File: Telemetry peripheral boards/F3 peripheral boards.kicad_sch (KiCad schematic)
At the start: 34 parts, among them J1 Hall Effect Sensor, J2 105313-1108, J3 Potentiometer, J4 Strain Gauge, U1 INA125U

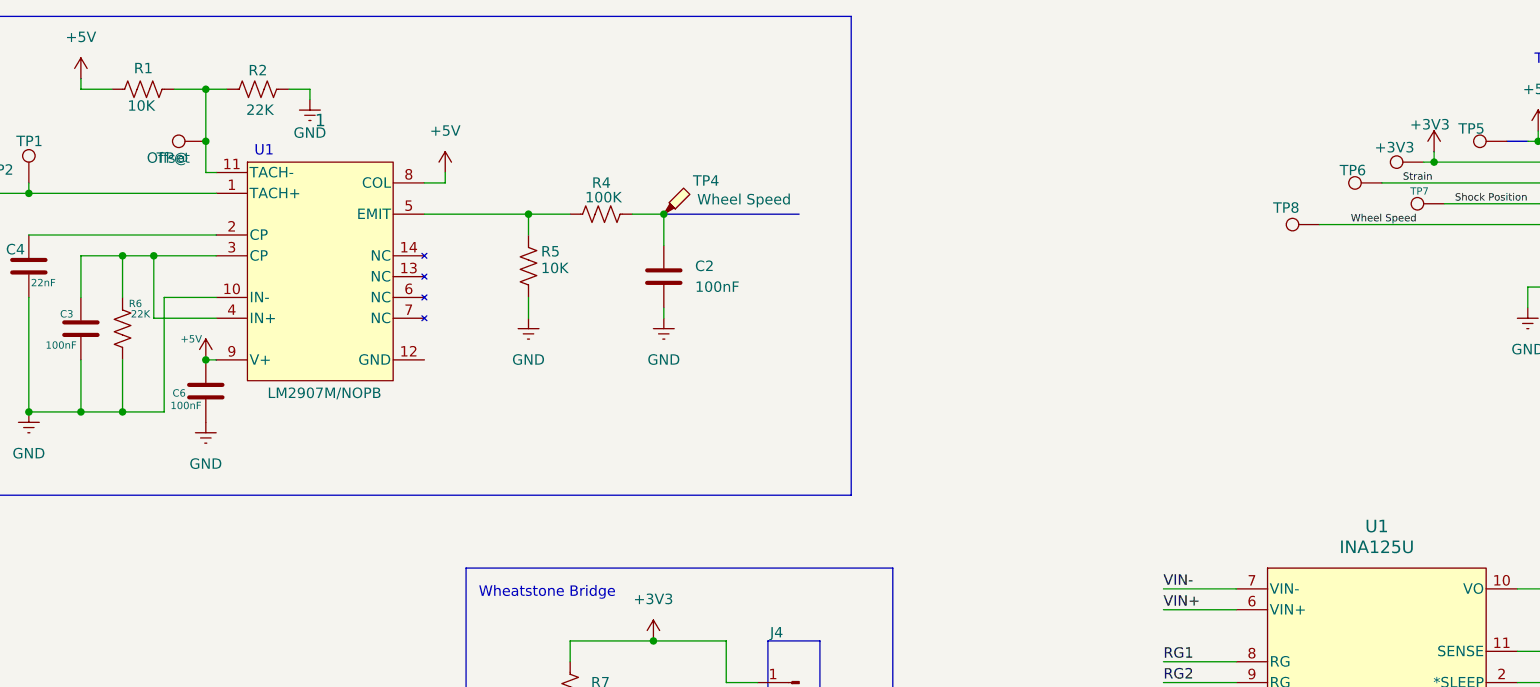
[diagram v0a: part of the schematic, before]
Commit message: Peripheral Board updates
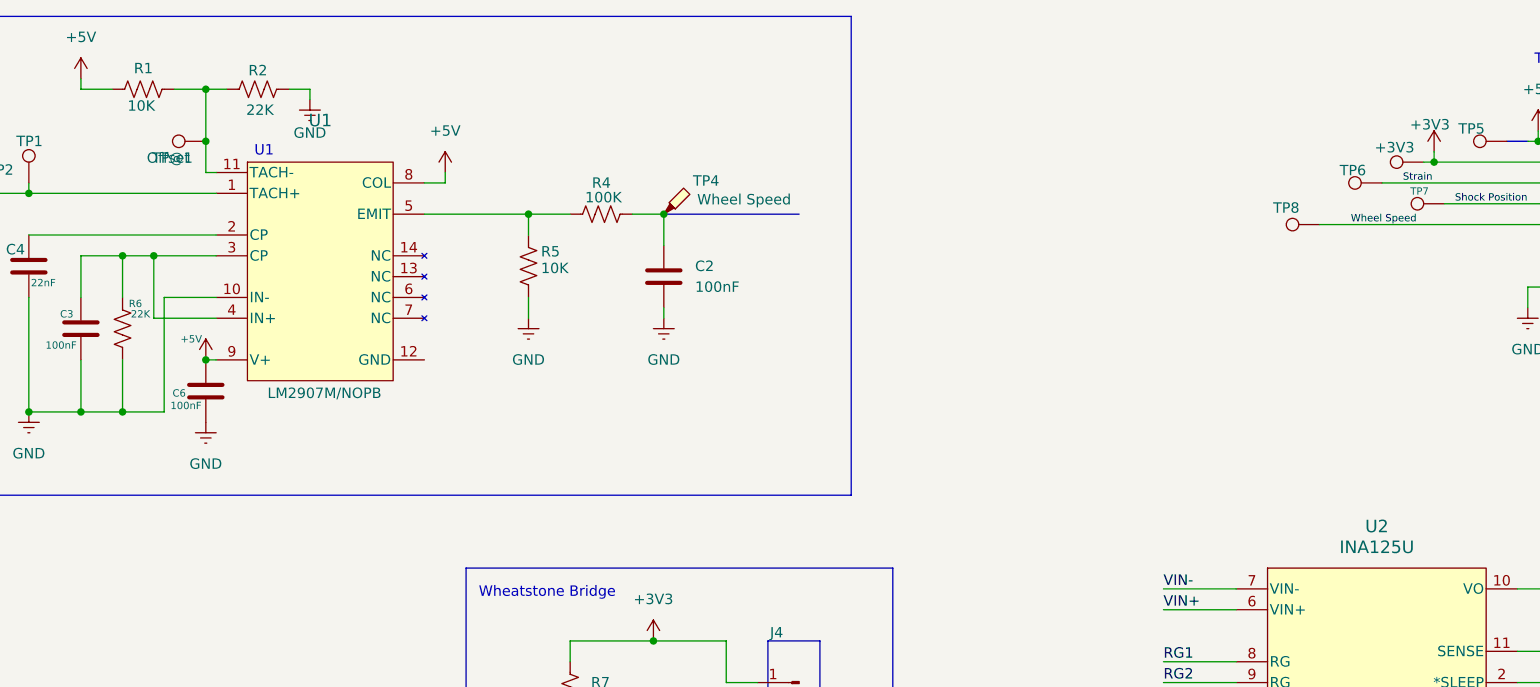
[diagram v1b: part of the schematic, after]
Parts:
- C1, C2, C3, C4, C5, C6: footprint (none) -> Capacitor_SMD:C_0805_2012Metric_Pad1.18x1.45mm_HandSolder
- R1, R10, R11, R2, R3, R4, R5, R6, R7, R8, R9: footprint (none) -> Resistor_SMD:R_0805_2012Metric_Pad1.20x1.40mm_HandSolder
- U1: renamed from 1; footprint (none) -> New Library:LM2907MNOPB
- U2: renamed from U1; footprint (none) -> New Library:105313-1108
- renumbered TP@ to TP@1
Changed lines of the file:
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@@
 			)
 		)
-		(property "Footprint" ""
+		(property "Footprint" "Resistor_SMD:R_0805_2012Metric_Pad1.20x1.40mm_HandSolder"
 			(at 94.234 30.734 90)
 			(effects
@@
 			)
 		)
-		(property "Footprint" ""
+		(property "Footprint" "Capacitor_SMD:C_0805_2012Metric_Pad1.18x1.45mm_HandSolder"
 			(at 73.3552 64.77 0)
 			(effects
@@
 			)
 		)
-		(property "Footprint" ""
+		(property "Footprint" "Resistor_SMD:R_0805_2012Metric_Pad1.20x1.40mm_HandSolder"
 			(at 78.486 61.214 90)
 			(effects
@@
 		(on_board yes)
 		(dnp no)
-		(property "Reference" "TP@"
+		(property "Reference" "TP@1"
 			(at 83.566 40.132 90)
 			(effects
@@
 			(project ""
 				(path "/dca14ea9-6ab5-4637-ab7d-1bf40ef85725"
-					(reference "TP@")
+					(reference "TP@1")
 					(unit 1)
 				)
@@
 			)
 		)
-		(property "Footprint" ""
+		(property "Footprint" "Capacitor_SMD:C_0805_2012Metric_Pad1.18x1.45mm_HandSolder"
 			(at 58.1152 57.15 0)
 			(effects
@@
 			)
 		)
-		(property "Footprint" ""
+		(property "Footprint" "Resistor_SMD:R_0805_2012Metric_Pad1.20x1.40mm_HandSolder"
 			(at 152.146 118.364 90)
 			(effects
@@
 			)
 		)
-		(property "Footprint" ""
+		(property "Footprint" "Resistor_SMD:R_0805_2012Metric_Pad1.20x1.40mm_HandSolder"
 			(at 44.196 52.324 90)
 			(effects
@@
 			)
 		)
-		(property "Footprint" ""
+		(property "Footprint" "Capacitor_SMD:C_0805_2012Metric_Pad1.18x1.45mm_HandSolder"
 			(at 67.0052 57.15 0)
 			(effects
@@
 		(dnp no)
 		(fields_autoplaced yes)
-		(property "Reference" "U1"
+		(property "Reference" "U2"
 			(at 230.505 85.09 0)
 			(effects
@@
 			)
 		)
-		(property "Footprint" ""
+		(property "Footprint" "New Library:105313-1108"
 			(at 200.66 95.25 0)
 			(effects
@@
 			(project ""
 				(path "/dca14ea9-6ab5-4637-ab7d-1bf40ef85725"
-					(reference "U1")
+					(reference "U2")
 					(unit 1)
 				)
@@
 			)
 		)
-		(property "Footprint" ""
+		(property "Footprint" "Resistor_SMD:R_0805_2012Metric_Pad1.20x1.40mm_HandSolder"
 			(at 136.144 45.974 90)
 			(effects
@@
 			)
 		)
-		(property "Footprint" ""
+		(property "Footprint" "Resistor_SMD:R_0805_2012Metric_Pad1.20x1.40mm_HandSolder"
 			(at 128.016 53.594 90)
 			(effects
@@
 			)
 		)
-		(property "Footprint" ""
+		(property "Footprint" "Resistor_SMD:R_0805_2012Metric_Pad1.20x1.40mm_HandSolder"
 			(at 133.096 118.364 90)
 			(effects
@@
 			)
 		)
-		(property "Footprint" ""
+		(property "Footprint" "Resistor_SMD:R_0805_2012Metric_Pad1.20x1.40mm_HandSolder"
 			(at 79.756 32.766 90)
 			(effects
@@
 			)
 		)
-		(property "Footprint" ""
+		(property "Footprint" "Capacitor_SMD:C_0805_2012Metric_Pad1.18x1.45mm_HandSolder"
 			(at 88.5952 72.39 0)
 			(effects
@@
 		(on_board yes)
 		(dnp no)
-		(property "Reference" "1"
+		(property "Reference" "U1"
 			(at 101.6 35.56 0)
 			(effects
@@
 			)
 		)
-		(property "Footprint" ""
+		(property "Footprint" "New Library:LM2907MNOPB"
 			(at 104.14 65.024 0)
 			(effects
@@
 			(project ""
 				(path "/dca14ea9-6ab5-4637-ab7d-1bf40ef85725"
-					(reference "1")
+					(reference "U1")
 					(unit 1)
 				)
@@
 			)
 		)
-		(property "Footprint" ""
+		(property "Footprint" "Resistor_SMD:R_0805_2012Metric_Pad1.20x1.40mm_HandSolder"
 			(at 133.096 105.664 90)
 			(effects
@@
 			)
 		)
-		(property "Footprint" ""
+		(property "Footprint" "Capacitor_SMD:C_0805_2012Metric_Pad1.18x1.45mm_HandSolder"
 			(at 207.9752 144.78 0)
 			(effects
@@
 			)
 		)
-		(property "Footprint" ""
+		(property "Footprint" "Resistor_SMD:R_0805_2012Metric_Pad1.20x1.40mm_HandSolder"
 			(at 116.586 151.384 90)
 			(effects
@@
 			)
 		)
-		(property "Footprint" ""
+		(property "Footprint" "Resistor_SMD:R_0805_2012Metric_Pad1.20x1.40mm_HandSolder"
 			(at 108.966 151.384 90)
 			(effects
@@
 			)
 		)
-		(property "Footprint" ""
+		(property "Footprint" "Capacitor_SMD:C_0805_2012Metric_Pad1.18x1.45mm_HandSolder"
 			(at 144.4752 58.42 0)
 			(effects

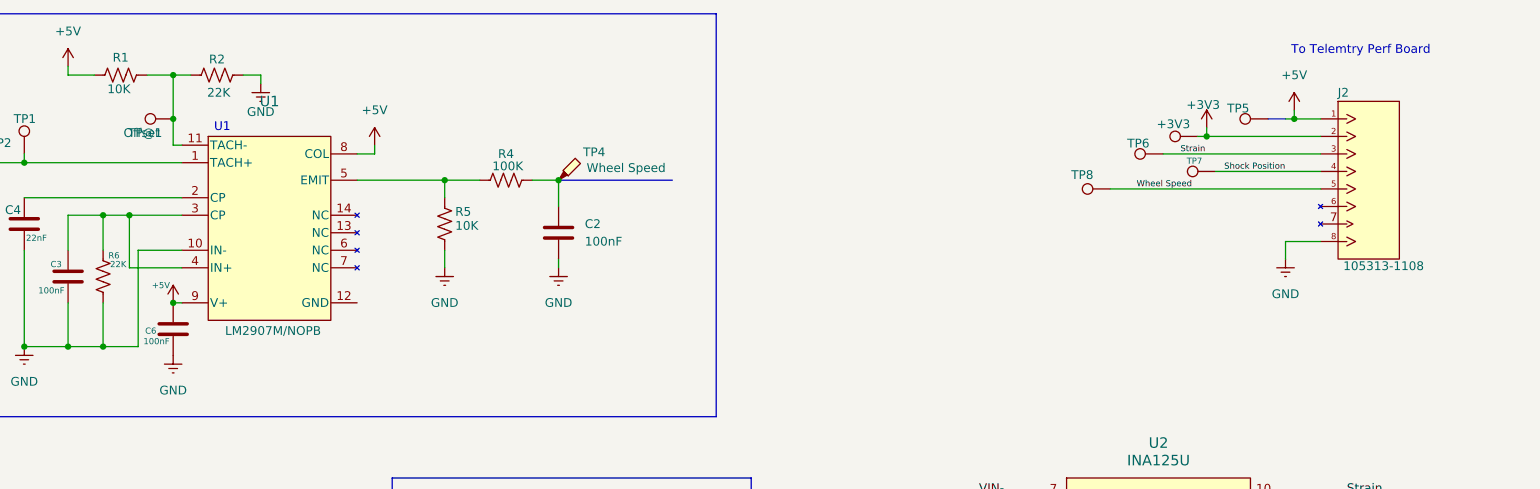
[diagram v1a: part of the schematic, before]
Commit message: Updates to peripheral boards
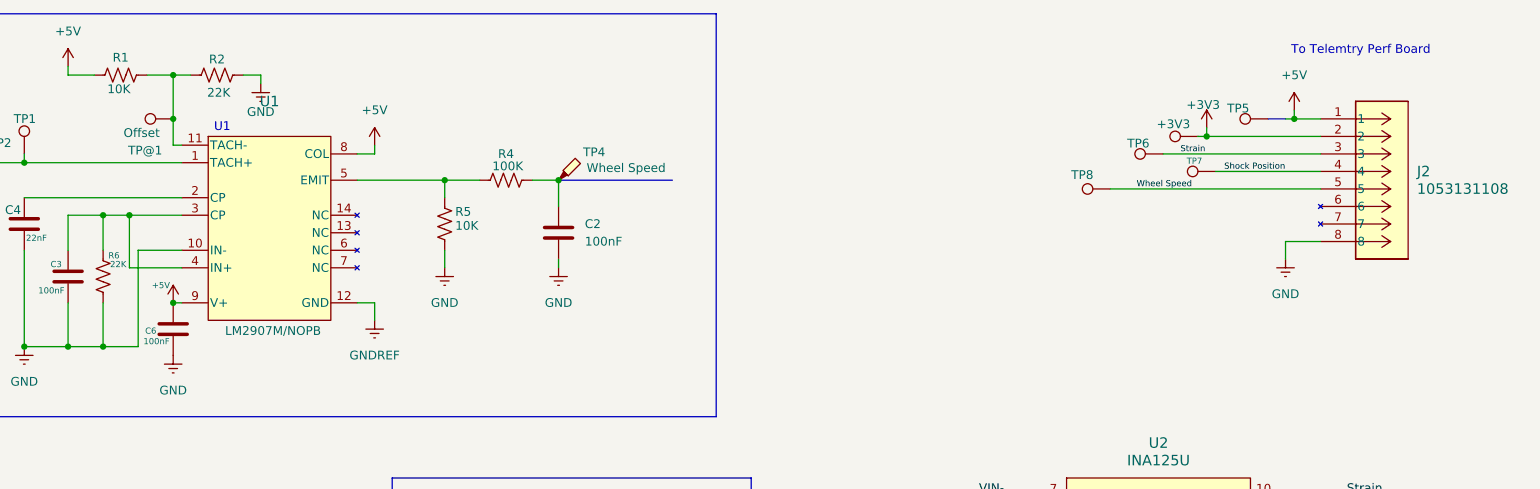
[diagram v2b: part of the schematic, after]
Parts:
- removed J2: 105313-1108, symbol Connector:Conn_01x08_Pin
- added J2: 1053131108, New Library:CON_1053131108, symbol New_Library:1053131108
- J1, J4: footprint (none) -> Connector_PinHeader_2.00mm:PinHeader_1x02_P2.00mm_Vertical
- J3: footprint (none) -> Potentiometer_SMD:Potentiometer_ACP_CA6-VSMD_Vertical
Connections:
- net +3V3: now also J2.2
- net +5V: now also J2.1
- net GND: now also J2.8
- net GNDREF: now also U1.12 (GND)
- net Shock Position: now also J2.4
- net Strain: now also J2.3
- net Wheel Speed: now also J2.5
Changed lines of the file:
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@@
 	(wire
 		(pts
+			(xy 116.84 64.77) (xy 114.3 64.77)
+		)
+		(stroke
+			(width 0)
+			(type default)
+		)
+	)
+	(wire
+		(pts
 			(xy 252.73 104.14) (xy 247.65 104.14)
 		)
@@
 	(wire
 		(pts
+			(xy 116.84 67.31) (xy 116.84 64.77)
+		)
+		(stroke
+			(width 0)
+			(type default)
+		)
+	)
+	(wire
+		(pts
 			(xy 132.08 124.46) (xy 142.24 124.46)
 		)
@@
 	)
 	(symbol
+		(lib_id "New_Library:1053131108")
+		(at 254 38.1 0)
+		(unit 1)
+		(exclude_from_sim no)
+		(in_bom yes)
+		(on_board yes)
+		(dnp no)
+		(fields_autoplaced yes)
+		(property "Reference" "J2"
+			(at 267.97 45.7199 0)
+			(effects
+				(font
+					(size 1.524 1.524)
+				)
+				(justify left)
+			)
+		)
+		(property "Value" "1053131108"
+			(at 267.97 48.2599 0)
+			(effects
+				(font
+					(size 1.524 1.524)
+				)
+				(justify left)
+			)
+		)
+		(property "Footprint" "New Library:CON_1053131108"
+			(at 259.842 34.544 0)
+			(effects
+				(font
+					(size 1.27 1.27)
+					(italic yes)
+				)
+				(hide yes)
+			)
+		)
+		(property "Datasheet" "1053131108"
+			(at 259.842 60.452 0)
+			(effects
+				(font
+					(size 1.27 1.27)
+					(italic yes)
+				)
+				(hide yes)
+			)
+		)
+		(property "Description" ""
+			(at 254 38.1 0)
+			(effects
+				(font
+					(size 1.27 1.27)
+				)
+				(hide yes)
+			)
+		)
+		(pin "6"
+		)
+		(pin "1"
+		)
+		(pin "2"
+		)
+		(pin "4"
+		)
+		(pin "5"
+		)
+		(pin "3"
+		)
+		(pin "8"
+		)
+		(pin "7"
+		)
+		(instances
+			(project ""
+				(path "/dca14ea9-6ab5-4637-ab7d-1bf40ef85725"
+					(reference "J2")
+					(unit 1)
+				)
+			)
+		)
+	)
+	(symbol
 		(lib_id "power:GNDREF")
 		(at 127 59.69 0)
@@
 		(dnp no)
 		(property "Reference" "TP@1"
-			(at 83.566 40.132 90)
+			(at 83.566 42.672 90)
 			(effects
 				(font
@@
 	)
 	(symbol
-		(lib_id "Connector:Conn_01x08_Pin")
-		(at 248.92 45.72 0)
-		(unit 1)
-		(exclude_from_sim no)
-		(in_bom yes)
-		(on_board yes)
-		(dnp no)
-		(property "Reference" "J2"
-			(at 257.302 34.29 0)
-			(effects
-				(font
-					(size 1.27 1.27)
-				)
-			)
-		)
-		(property "Value" "105313-1108"
-			(at 263.144 59.436 0)
-			(effects
-				(font
-					(size 1.27 1.27)
-				)
-			)
-		)
-		(property "Footprint" ""
-			(at 248.92 45.72 0)
-			(effects
-				(font
-					(size 1.27 1.27)
-				)
-				(hide yes)
-			)
-		)
-		(property "Datasheet" ""
-			(at 248.92 45.72 0)
-			(effects
-				(font
-					(size 1.27 1.27)
-				)
-				(hide yes)
-			)
-		)
-		(property "Description" ""
-			(at 248.92 45.72 0)
-			(effects
-				(font
-					(size 1.27 1.27)
-				)
-				(hide yes)
-			)
-		)
-		(pin "1"
-		)
-		(pin "2"
-		)
-		(pin "8"
-		)
-		(pin "7"
-		)
-		(pin "3"
-		)
-		(pin "4"
-		)
-		(pin "6"
-		)
-		(pin "5"
-		)
-		(instances
-			(project ""
-				(path "/dca14ea9-6ab5-4637-ab7d-1bf40ef85725"
-					(reference "J2")
-					(unit 1)
-				)
-			)
-		)
-	)
-	(symbol
 		(lib_id "Connector:TestPoint")
 		(at 223.52 48.26 90)
@@
 			)
 		)
-		(property "Footprint" ""
+		(property "Footprint" "Connector_PinHeader_2.00mm:PinHeader_1x02_P2.00mm_Vertical"
 			(at 160.02 106.68 0)
 			(effects
@@
 			)
 		)
-		(property "Footprint" ""
+		(property "Footprint" "Connector_PinHeader_2.00mm:PinHeader_1x02_P2.00mm_Vertical"
 			(at 29.21 41.91 0)
 			(effects
@@
 	)
 	(symbol
+		(lib_id "power:GNDREF")
+		(at 116.84 67.31 0)
+		(unit 1)
+		(exclude_from_sim no)
+		(in_bom yes)
+		(on_board yes)
+		(dnp no)
+		(fields_autoplaced yes)
+		(property "Reference" "#PWR023"
+			(at 116.84 73.66 0)
+			(effects
+				(font
+					(size 1.27 1.27)
+				)
+				(hide yes)
+			)
+		)
+		(property "Value" "GNDREF"
+			(at 116.84 72.39 0)
+			(effects
+				(font
+					(size 1.27 1.27)
+				)
+			)
+		)
+		(property "Footprint" ""
+			(at 116.84 67.31 0)
+			(effects
+				(font
+					(size 1.27 1.27)
+				)
+				(hide yes)
+			)
+		)
+		(property "Datasheet" ""
+			(at 116.84 67.31 0)
+			(effects
+				(font
+					(size 1.27 1.27)
+				)
+				(hide yes)
+			)
+		)
+		(property "Description" "Power symbol creates a global label with name \"GNDREF\" , reference supply ground"
+			(at 116.84 67.31 0)
+			(effects
+				(font
+					(size 1.27 1.27)
+				)
+				(hide yes)
+			)
+		)
+		(pin "1"
+		)
+		(instances
+			(project ""
+				(path "/dca14ea9-6ab5-4637-ab7d-1bf40ef85725"
+					(reference "#PWR023")
+					(unit 1)
+				)
+			)
+		)
+	)
+	(symbol
 		(lib_id "Device:C")
 		(at 143.51 54.61 0)
@@
 			)
 		)
-		(property "Footprint" ""
+		(property "Footprint" "Potentiometer_SMD:Potentiometer_ACP_CA6-VSMD_Vertical"
 			(at 31.75 99.06 0)
 			(effects
